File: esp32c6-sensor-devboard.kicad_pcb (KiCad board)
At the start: 4 copper layers, 183 parts, among them J1 Conn_01x04_Pin, J2 Micro_SD_Card_Det1, J3 Screw_Terminal_01x02, J4 USB_C_Receptacle_USB2.0_14P, J5 Screw_Terminal_01x02, J6 Screw_Terminal_01x06, J7 Screw_Terminal_01x04, J8 Conn_01x04_Pin, J9 Conn_01x03_Pin, SW1 SW_Push, SW2 SW_Push, SW3 SW_DIP_x04, U1 ESP32-C6, U10 LM393, U11 TCA9555RTWR, U12 LM393, U13 LM393, U14 TMP117AIDRV, U15 BMP581, U16 TMP117AIDRV, U2 W25Q128JVS, U3 AP2112K-3.3, U4 LM317_TO-252, U5 LMR36520FADDA, U6 CJ431, U7 USBLC6-2SC6, U8 CJ431, U9 LMR36520FADDA, Y1 48M, Y2 32k768

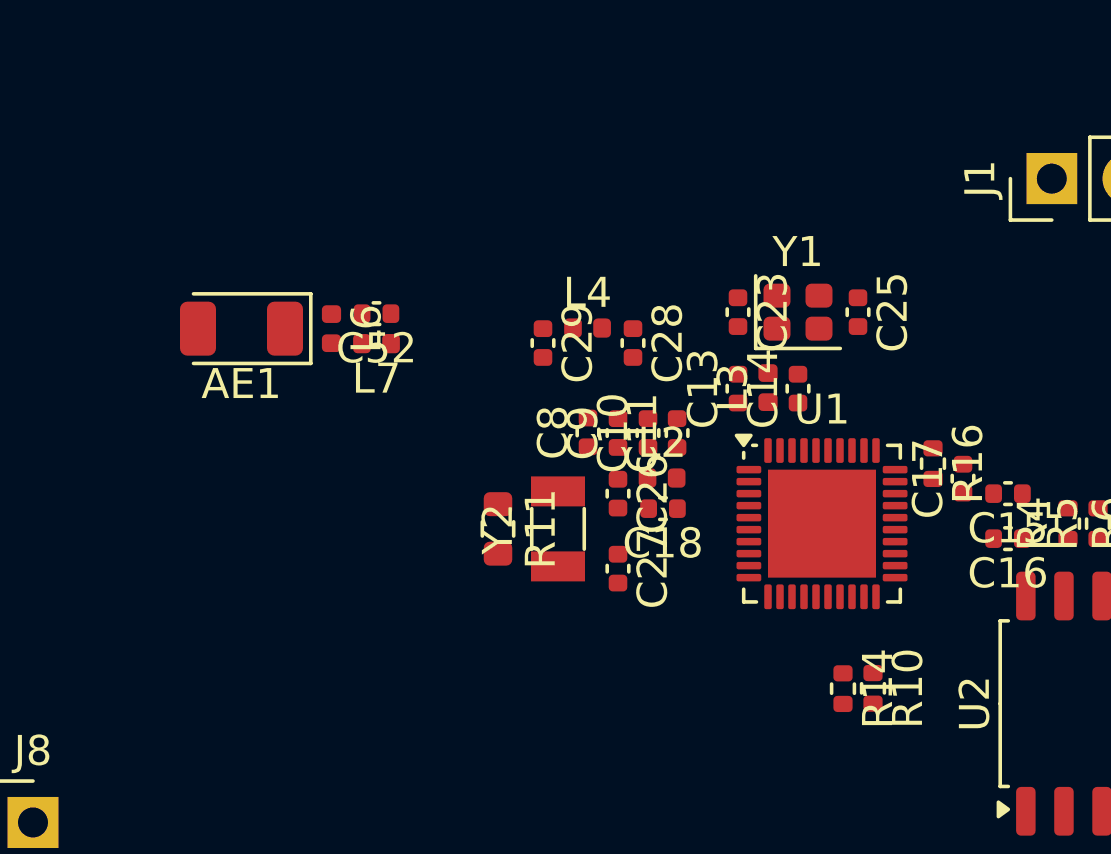
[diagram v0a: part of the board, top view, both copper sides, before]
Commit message: pcb: rf layout
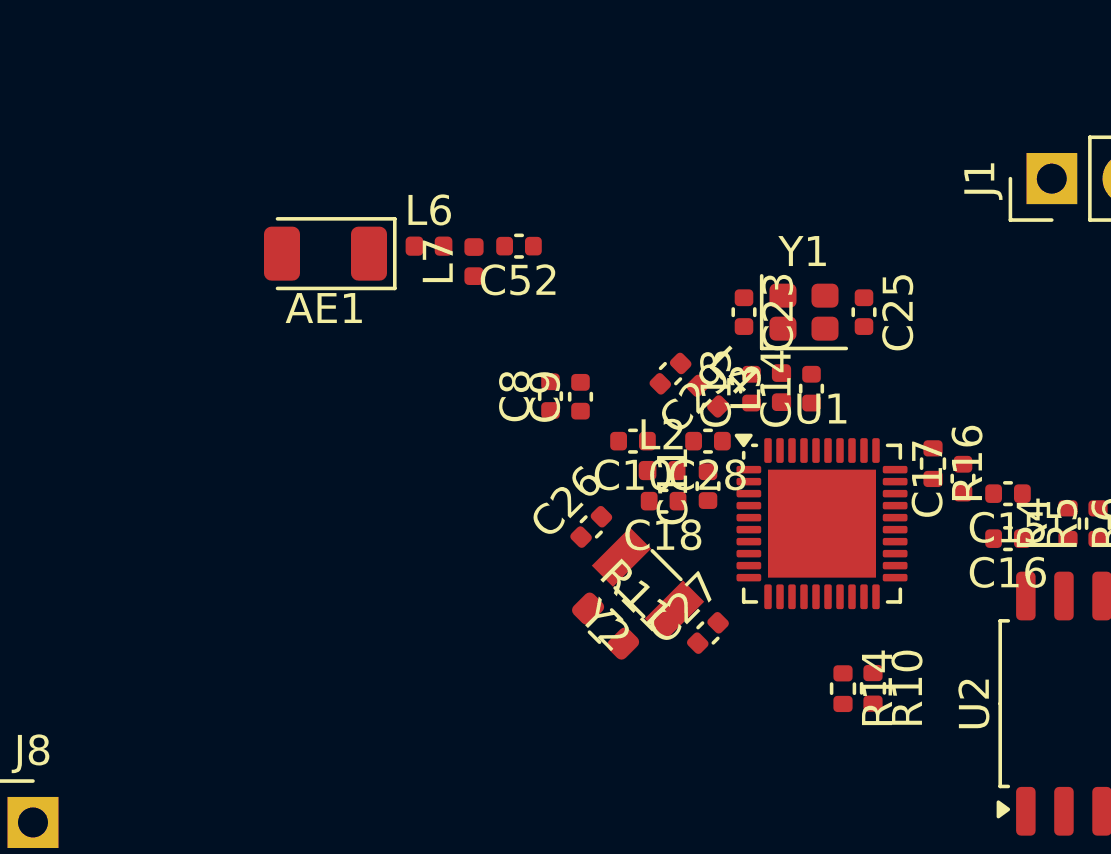
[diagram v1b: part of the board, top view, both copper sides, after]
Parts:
- moved C52 5.26 mm to (138.7, 85.2)
- moved R11 4.83 mm to (141.6, 97.9), turned to -45 degrees
- moved L4 4.61 mm to (145.0, 90.2), turned to -45 degrees
- moved C29 4.37 mm to (143.8, 89.5), turned to -135 degrees
- moved L6 4.26 mm to (135.7, 85.2), turned to 0 degrees
- moved L7 4.25 mm to (137.2, 85.8), turned to 90 degrees
- moved C28 4.12 mm to (145.0, 91.8), turned to 180 degrees
- moved AE1 3.75 mm to (132.2, 85.5)
- moved C27 3.69 mm to (145.0, 98.1), turned to 45 degrees
- moved Y2 3.51 mm to (143.0, 96.5), turned to 135 degrees
- moved C11 2.05 mm to (145.0, 93.2)
- moved C9 1.74 mm to (140.8, 90.3)
- moved C8 1.74 mm to (139.8, 90.2)
- moved C26 1.42 mm to (141.1, 94.6), turned to 45 degrees
- moved C10 0.57 mm to (142.5, 91.8), turned to 180 degrees
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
